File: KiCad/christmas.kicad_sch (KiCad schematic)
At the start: 23 parts, among them J1 Conn_01x03, J2 Conn_01x03, U4 74HC595

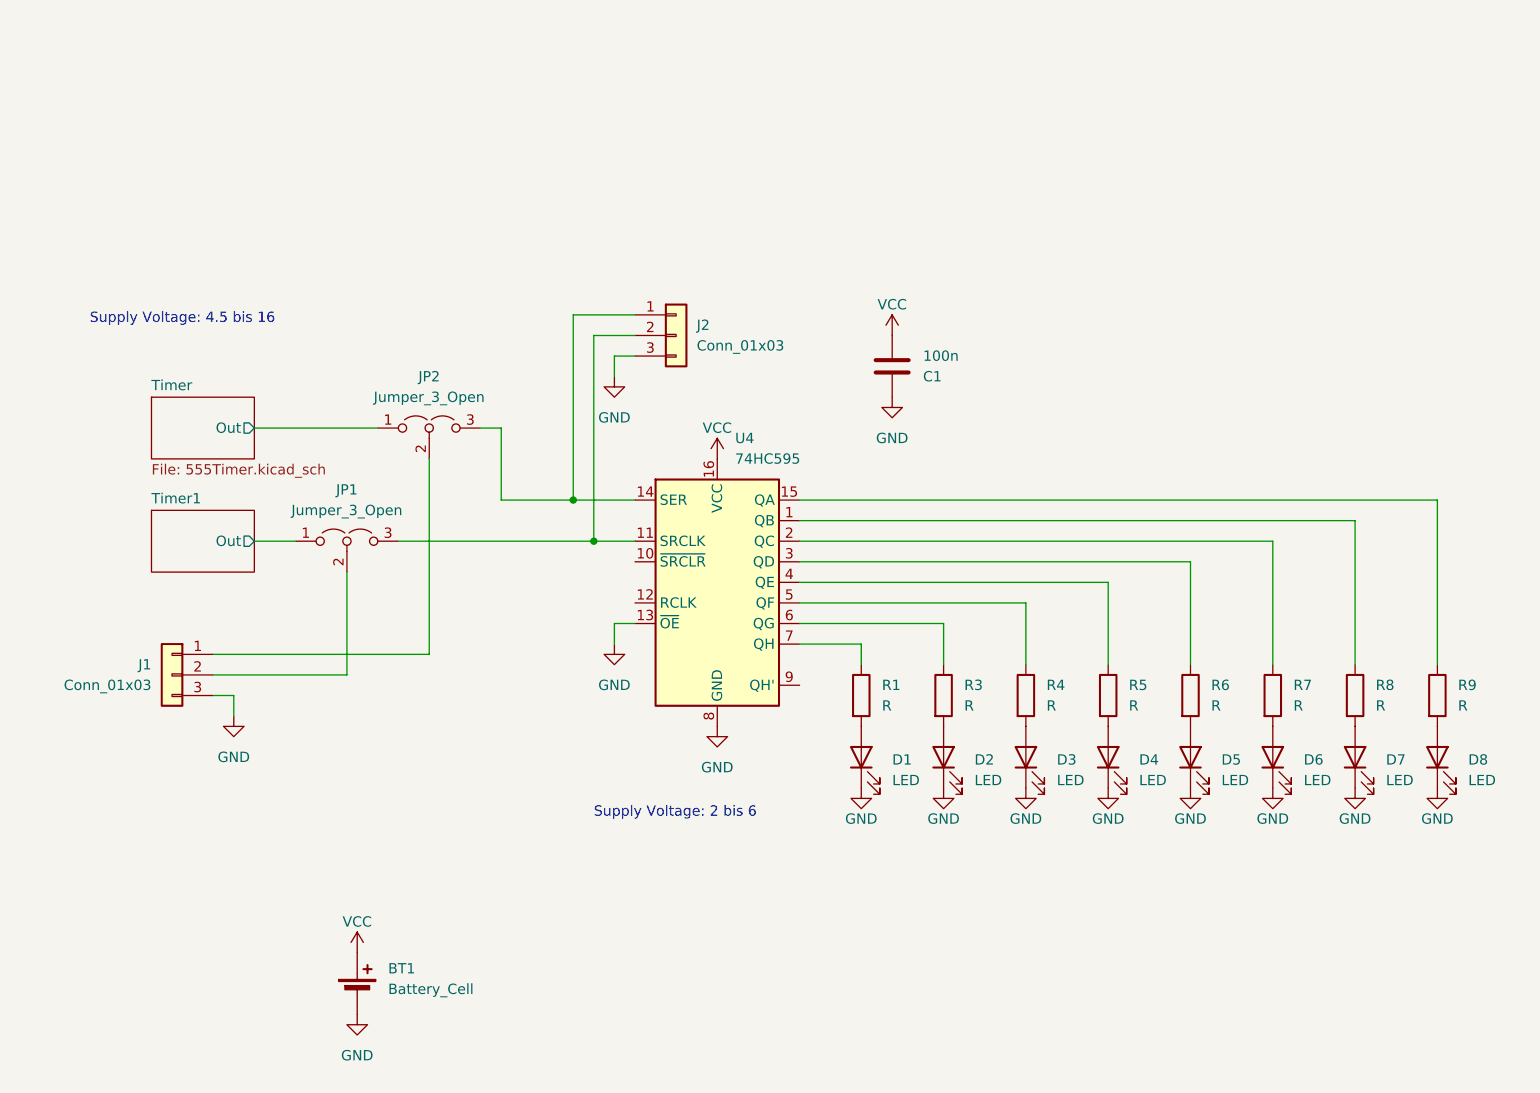
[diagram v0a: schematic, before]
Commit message: minor fixes
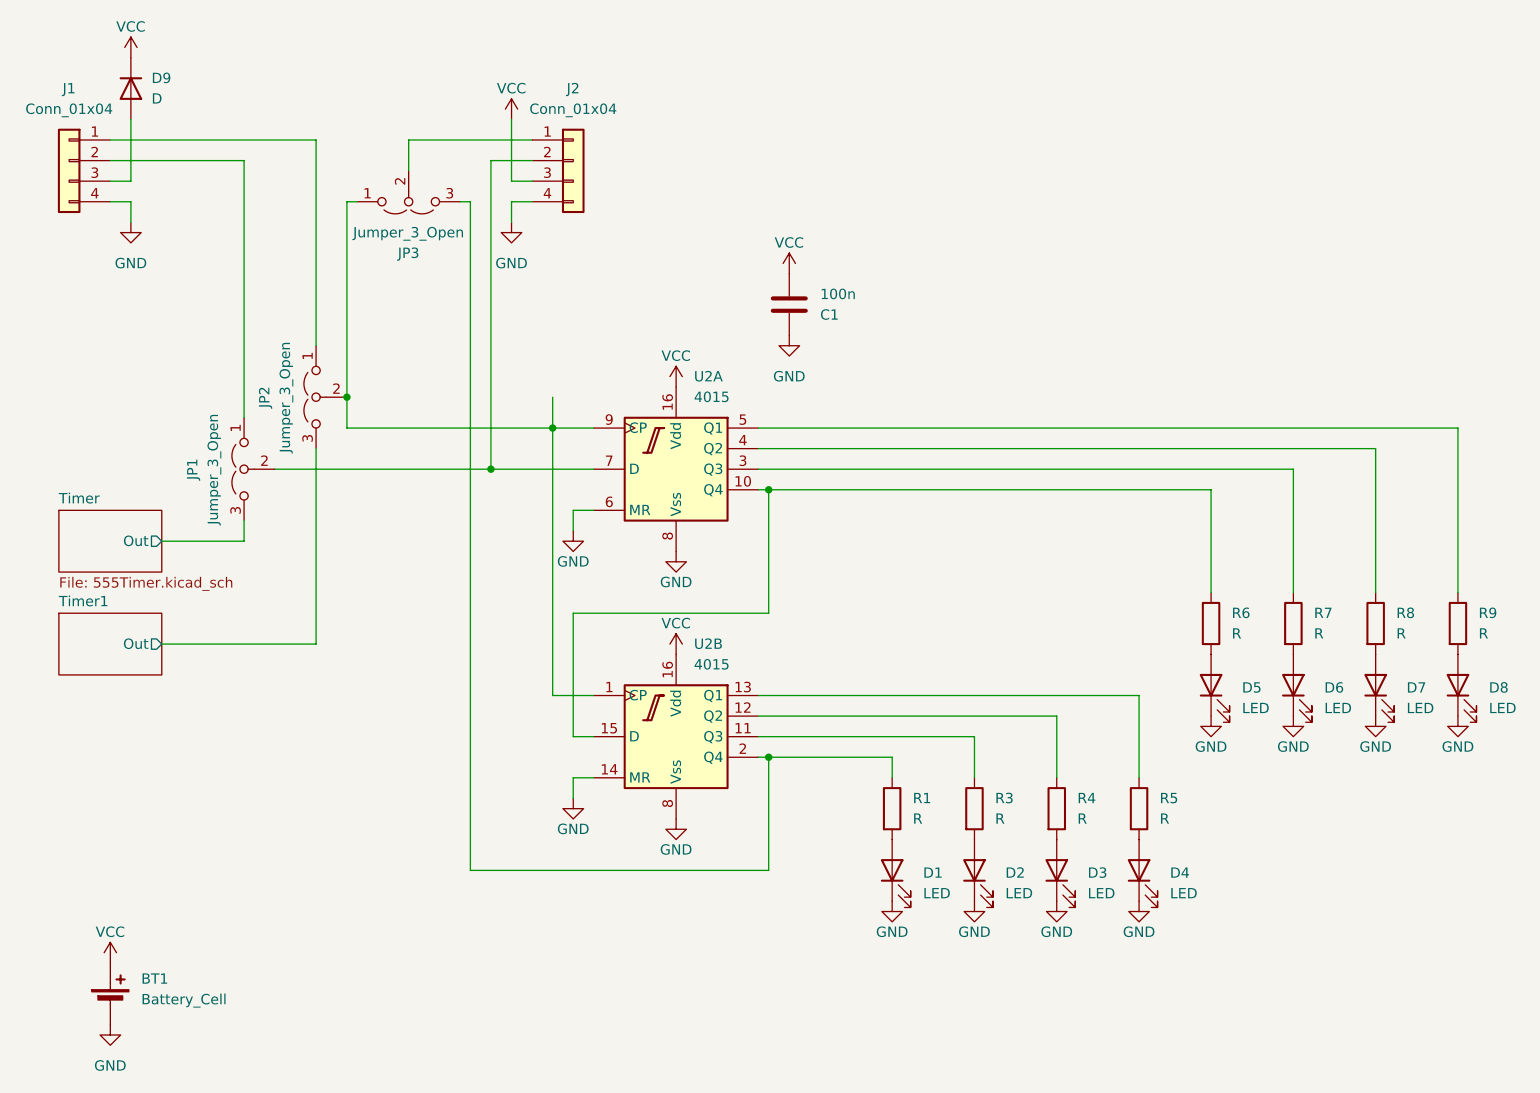
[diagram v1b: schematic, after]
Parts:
- removed J1, J2: Conn_01x03, Connector_PinHeader_2.54mm:PinHeader_1x03_P2.54mm_Vertical, symbol Connector_Generic:Conn_01x03
- removed U4: 74HC595, symbol 74xx:74HC595
- added D9: D, symbol Device:D
- added J1, J2: Conn_01x04, Connector_Molex:Molex_KK-254_AE-6410-04A_1x04_P2.54mm_Vertical, symbol Connector_Generic:Conn_01x04
- added JP3: Jumper_3_Open, Connector_PinHeader_2.54mm:PinHeader_1x03_P2.54mm_Vertical, symbol Jumper:Jumper_3_Open
- added U2: 4015, Package_DIP:DIP-16_W10.16mm_LongPads, symbol 4xxx_IEEE:4015
- C1: footprint (none) -> Capacitor_THT:C_Disc_D5.0mm_W2.5mm_P5.00mm
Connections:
- net GND: now also J1.4 (Pin_4), J2.4 (Pin_4), U2.14 (MR), U2.6 (MR), U2.8 (Vss), U2.8 (Vss)
- net Timer/Out: now also JP1.3 (B); no longer JP2.1 (A)
- net Timer1/Out: now also JP2.3 (B); no longer JP1.1 (A)
- net VCC: now also D9.1 (K), J2.3 (Pin_3), U2.16 (Vdd), U2.16 (Vdd)
- net at R7.1: now also U2.3 (Q3)
- net at JP2.2 (C): now also JP3.1 (A), U2.1 (CP), U2.9 (CP)
- net at JP1.2 (C): now also J2.2 (Pin_2), U2.7 (D)
- net at R1.1: now also JP3.3 (B), U2.2 (Q4)
- net at R9.1: now also U2.5 (Q1)
- net at R4.1: now also U2.12 (Q2)
- net at R8.1: now also U2.4 (Q2)
- net at R6.1: now also U2.10 (Q4), U2.15 (D)
- net at R5.1: now also U2.13 (Q1)
- net at R3.1: now also U2.11 (Q3)
- new net: J2.1 (Pin_1), JP3.2 (C)
- new net: J1.1 (Pin_1), JP2.1 (A)
- new net: J1.2 (Pin_2), JP1.1 (A)
- new net: D9.2 (A), J1.3 (Pin_3)
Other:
- note removed: "Supply Voltage: 2 bis 6"
- note removed: "Supply Voltage: 4.5 bis 16"
- moved on the sheet: BT1, C1, D1, D2, D3, D4, D5, D6, D7, D8, JP1, JP2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
